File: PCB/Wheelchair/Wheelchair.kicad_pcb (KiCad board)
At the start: 2 copper layers, 57 x 67 mm, 24 parts, among them J1 Conn_01x04_Socket, J2 10118193-0001LF, J3 10118193-0001LF, J4 Conn_01x06_Pin, J5 Conn_01x09_Pin, SW1 SW_MEC_5E, U1 MC14069UBCPG, U2 CP2102N-A02-GQFN20

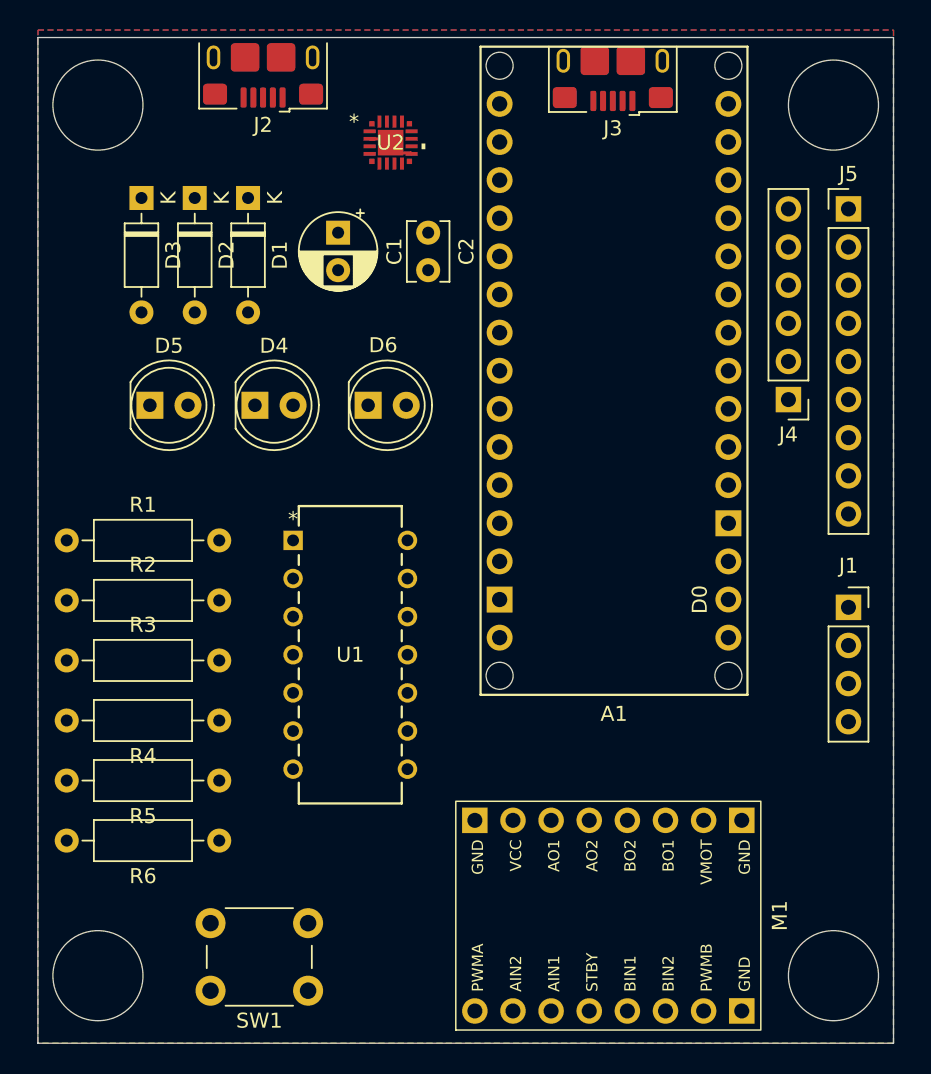
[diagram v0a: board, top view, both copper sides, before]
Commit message: PCB_routed
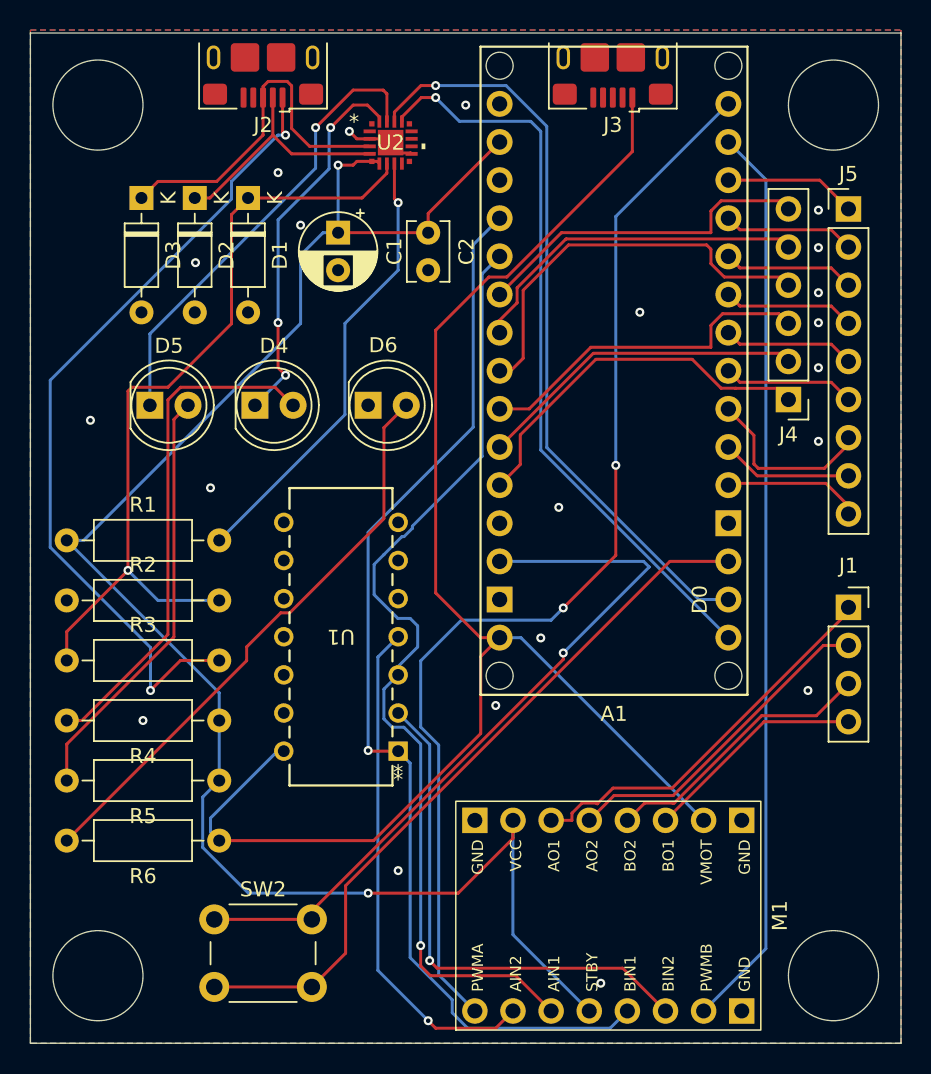
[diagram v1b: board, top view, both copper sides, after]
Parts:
- removed SW1: SW_MEC_5E, Button_Switch_THT:SW_PUSH_6mm_H4.3mm
- added SW2: SW_Push_Open_Dual, Button_Switch_THT:SW_PUSH_6mm_H4.3mm, F.Cu at (196.8, 108.2)
- moved U1 15.7 mm to (209.0, 97.0), turned to 180 degrees
- moved J3 0.22 mm to (223.3, 50.8)
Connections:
- J2 pad 6: GND -> (no net)
- J3 pad 6: GND -> (no net)
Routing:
- net +3.3V: track 0.00 -> 115.2 mm, vias 0 -> 2
- net +5V: track 0.00 -> 99.0 mm
- net PWMA: track 0.00 -> 73.9 mm, vias 0 -> 2
- net DirB: track 0.00 -> 72.6 mm, vias 0 -> 1
- net DirA: track 0.00 -> 64.8 mm, vias 0 -> 1
- net PWMB: track 0.00 -> 60.6 mm
- net Net-(D1-K): track 0.00 -> 54.7 mm, vias 0 -> 1
- net USB_VBUS: track 0.00 -> 54.6 mm, vias 0 -> 2
- net RX: track 0.00 -> 50.3 mm, vias 0 -> 1
- net TX: track 0.00 -> 49.9 mm, vias 0 -> 1
- net Net-(A1-RESET-PadRST2): track 0.00 -> 49.4 mm, vias 0 -> 1
- net Net-(A1-RESET-PadRST1): track 0.00 -> 48.6 mm
- net Net-(D6-A): track 0.00 -> 38.7 mm
- net !DirB: track 0.00 -> 34.5 mm, vias 0 -> 1
- net Net-(D4-A): track 0.00 -> 33.9 mm
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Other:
- board size 57 x 67 mm -> 58 x 67.3 mm
